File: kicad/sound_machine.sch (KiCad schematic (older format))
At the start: 17 parts, among them J1 Conn_01x02, J10 Conn_01x01, J11 Conn_01x01, J12 Conn_01x01, J2 Conn_01x15, J3 Conn_01x15, J4 TEST_1P, J5 Audio-Jack-3, J6 TEST_1P, J7 TEST_1P, J8 TEST_1P, J9 Conn_01x01, U1 MPU-6050_breakout, U2 DFPlayerMini

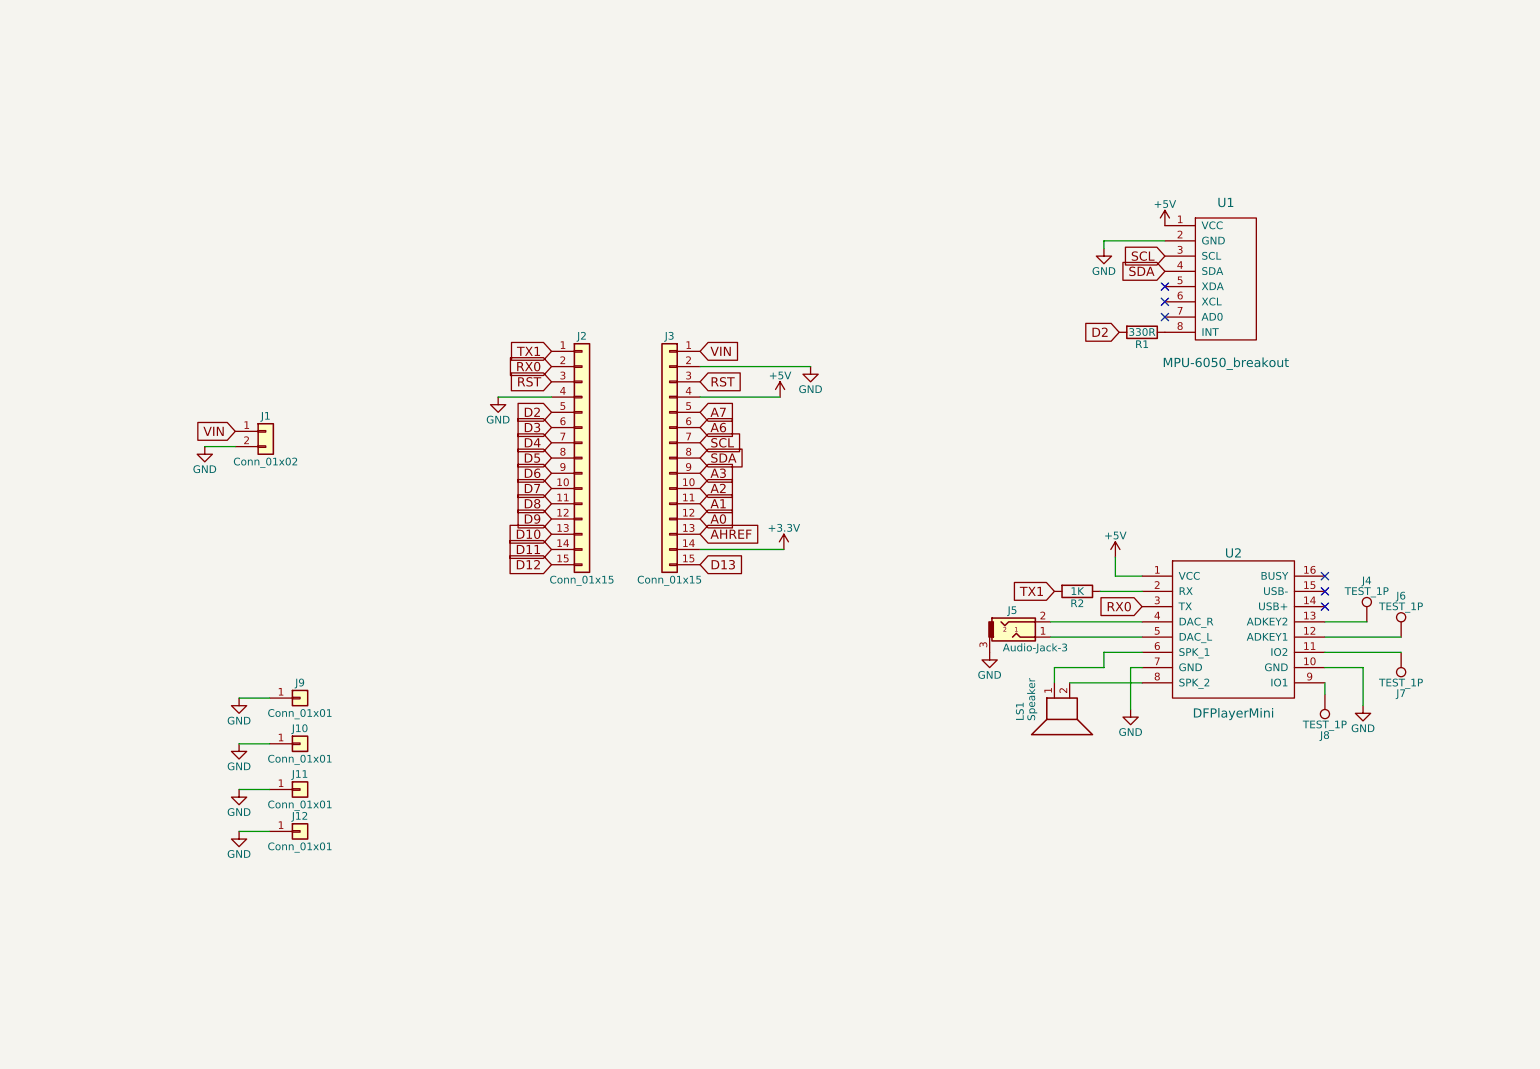
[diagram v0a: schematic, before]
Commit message: Nano expansion
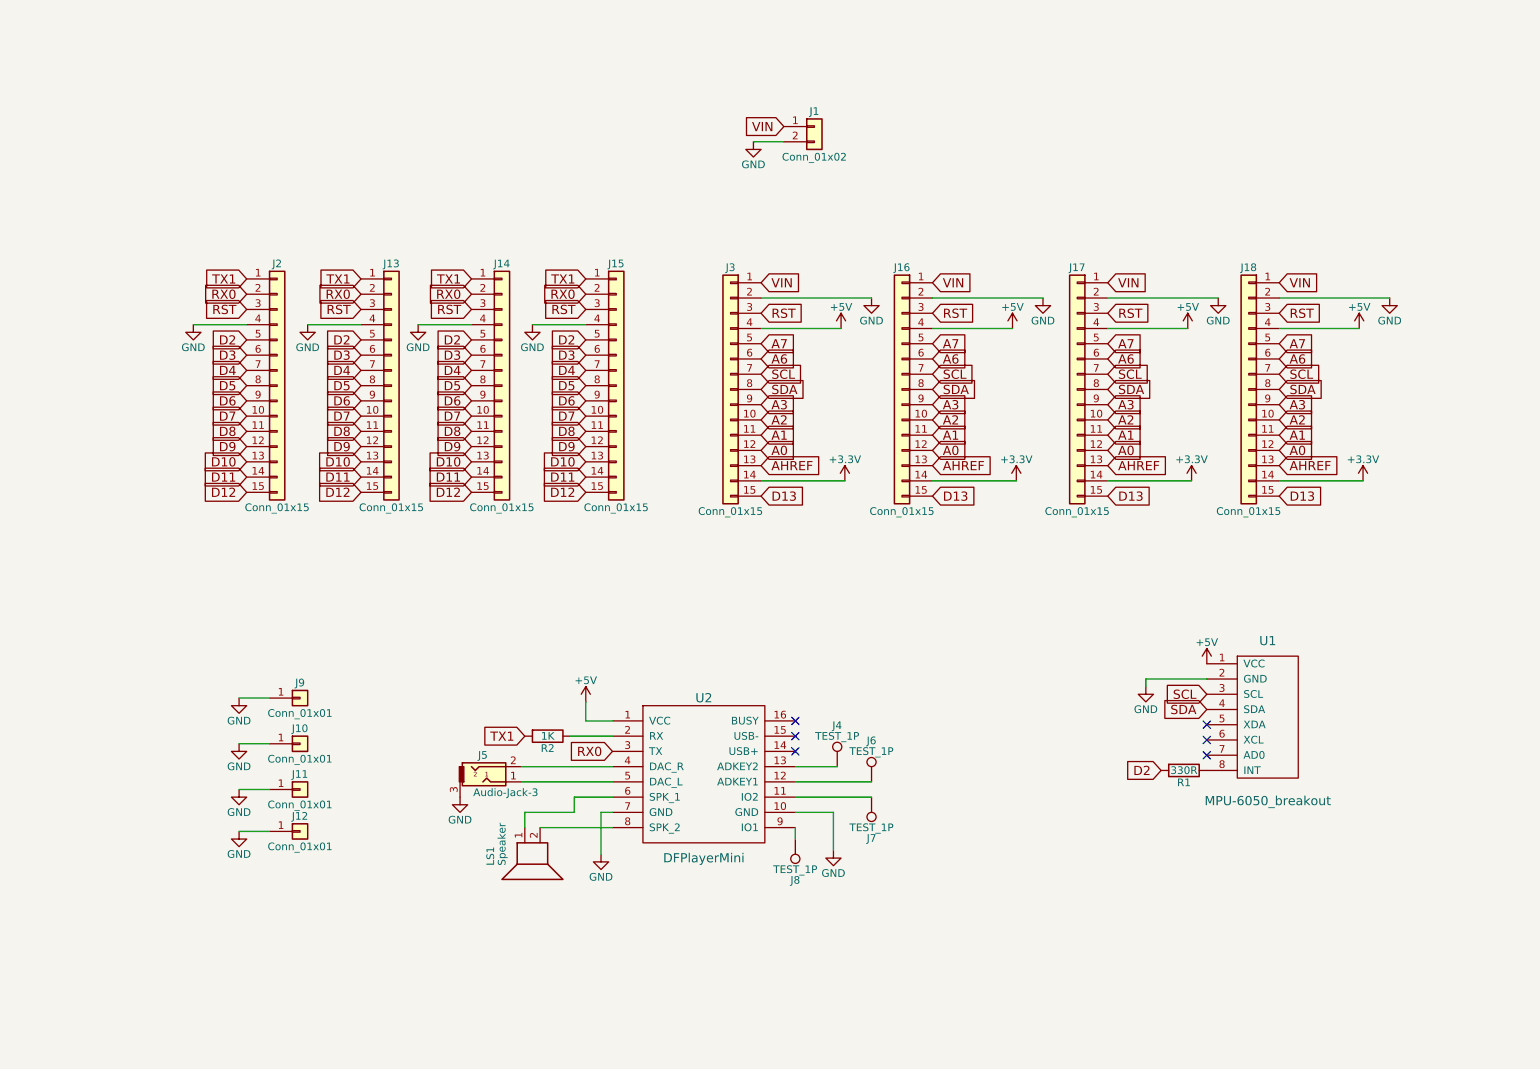
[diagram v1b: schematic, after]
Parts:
- added J13, J14, J15, J16, J17, J18: Conn_01x15, Pin_Headers:Pin_Header_Straight_1x15_Pitch2.54mm, symbol Conn_01x15
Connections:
- net +3V3: now also J16.14 (Pin_14), J17.14 (Pin_14), J18.14 (Pin_14)
- net +5V: now also J16.4 (Pin_4), J17.4 (Pin_4), J18.4 (Pin_4)
- net A0: now also J16.12 (Pin_12), J17.12 (Pin_12), J18.12 (Pin_12)
- net A1: now also J16.11 (Pin_11), J17.11 (Pin_11), J18.11 (Pin_11)
- net A2: now also J16.10 (Pin_10), J17.10 (Pin_10), J18.10 (Pin_10)
- net A3: now also J16.9 (Pin_9), J17.9 (Pin_9), J18.9 (Pin_9)
- net A6: now also J16.6 (Pin_6), J17.6 (Pin_6), J18.6 (Pin_6)
- net A7: now also J16.5 (Pin_5), J17.5 (Pin_5), J18.5 (Pin_5)
- net AHREF: now also J16.13 (Pin_13), J17.13 (Pin_13), J18.13 (Pin_13)
- net D10: now also J13.13 (Pin_13), J14.13 (Pin_13), J15.13 (Pin_13)
- net D11: now also J13.14 (Pin_14), J14.14 (Pin_14), J15.14 (Pin_14)
- net D12: now also J13.15 (Pin_15), J14.15 (Pin_15), J15.15 (Pin_15)
- net D13: now also J16.15 (Pin_15), J17.15 (Pin_15), J18.15 (Pin_15)
- net D2: now also J13.5 (Pin_5), J14.5 (Pin_5), J15.5 (Pin_5)
- net D3: now also J13.6 (Pin_6), J14.6 (Pin_6), J15.6 (Pin_6)
- net D4: now also J13.7 (Pin_7), J14.7 (Pin_7), J15.7 (Pin_7)
- net D5: now also J13.8 (Pin_8), J14.8 (Pin_8), J15.8 (Pin_8)
- net D6: now also J13.9 (Pin_9), J14.9 (Pin_9), J15.9 (Pin_9)
- net D7: now also J13.10 (Pin_10), J14.10 (Pin_10), J15.10 (Pin_10)
- net D8: now also J13.11 (Pin_11), J14.11 (Pin_11), J15.11 (Pin_11)
- net D9: now also J13.12 (Pin_12), J14.12 (Pin_12), J15.12 (Pin_12)
- net GND: now also J13.4 (Pin_4), J14.4 (Pin_4), J15.4 (Pin_4), J16.2 (Pin_2), J17.2 (Pin_2), J18.2 (Pin_2)
- net RST: now also J13.3 (Pin_3), J14.3 (Pin_3), J15.3 (Pin_3), J16.3 (Pin_3), J17.3 (Pin_3), J18.3 (Pin_3)
- net RX0: now also J13.2 (Pin_2), J14.2 (Pin_2), J15.2 (Pin_2)
- net SCL: now also J16.7 (Pin_7), J17.7 (Pin_7), J18.7 (Pin_7)
- net SDA: now also J16.8 (Pin_8), J17.8 (Pin_8), J18.8 (Pin_8)
- net TX1: now also J13.1 (Pin_1), J14.1 (Pin_1), J15.1 (Pin_1)
- net VIN: now also J16.1 (Pin_1), J17.1 (Pin_1), J18.1 (Pin_1)
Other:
- moved on the sheet: J1, J2, J3, J4, J5, J6, J7, J8, LS1, R1, R2, U1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

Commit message: Connected
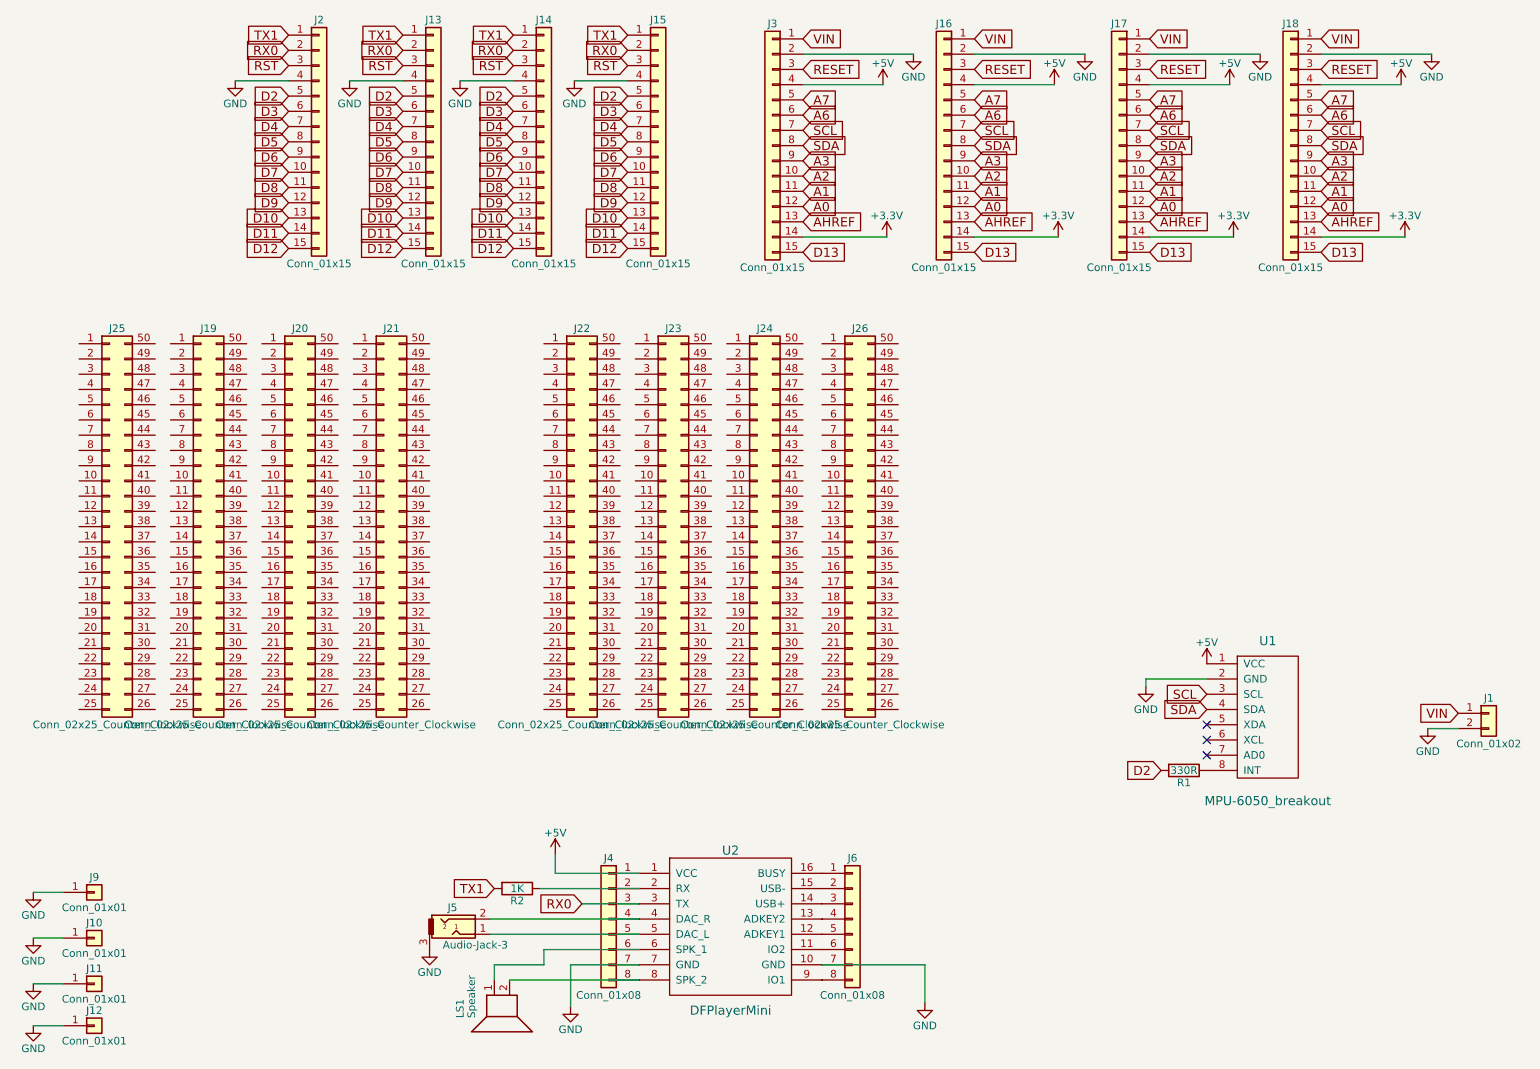
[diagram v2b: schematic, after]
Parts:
- removed J4, J6, J7, J8: TEST_1P, Measurement_Points:Measurement_Point_Round-SMD-Pad_Small, symbol TEST_1P
- added J19, J20, J21, J22, J23, J24, J25, J26: Conn_02x25_Counter_Clockwise, Pin_Headers:Pin_Header_Straight_2x25_Pitch2.54mm, symbol Conn_02x25_Counter_Clockwise
- added J4, J6: Conn_01x08, Pin_Headers:Pin_Header_Straight_1x08_Pitch2.54mm, symbol Conn_01x08
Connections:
- net +5V: now also J4.1 (Pin_1)
- net GND: now also J4.7 (Pin_7), J6.7 (Pin_7)
- net RST: no longer J16.3 (Pin_3), J17.3 (Pin_3), J18.3 (Pin_3), J3.3 (Pin_3)
- net RX0: now also J4.3 (Pin_3)
- net at U2.11 (IO2): now also J6.6 (Pin_6)
- net at U2.12 (ADKEY1): now also J6.5 (Pin_5)
- net at U2.13 (ADKEY2): now also J6.4 (Pin_4)
- net at U2.14 (USB+): now also J6.3 (Pin_3)
- net at U2.15 (USB-): now also J6.2 (Pin_2)
- net at U2.16 (BUSY): now also J6.1 (Pin_1)
- net at R2.1, U2.2 (RX): now also J4.2 (Pin_2)
- net at J5.2, U2.4 (DAC_R): now also J4.4 (Pin_4)
- net at J5.1, U2.5 (DAC_L): now also J4.5 (Pin_5)
- net at LS1.1, U2.6 (SPK_1): now also J4.6 (Pin_6)
- net at LS1.2, U2.8 (SPK_2): now also J4.8 (Pin_8)
- net at U2.9 (IO1): now also J6.8 (Pin_8)
- new net RESET: J16.3 (Pin_3), J17.3 (Pin_3), J18.3 (Pin_3), J3.3 (Pin_3)
- no-connect marks 6 -> 3
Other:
- moved on the sheet: J1, J10, J11, J12, J13, J14, J15, J16, J17, J18, J2, J3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
